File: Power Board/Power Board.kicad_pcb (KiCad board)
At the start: 2 copper layers, 55 x 70 mm, 147 parts, among them J1 Conn_02x07_Odd_Even, J2 Screw_Terminal_01x06, J3 Conn_01x03, J4 Conn_01x02, J5 Conn_02x03_Odd_Even, Q1 SI7157DP, Q2 SI7157DP, Q3 SI7157DP, Q4 SI7157DP, Q5 SI7157DP, Q6 SI7157DP, Q7 DMG2305UX, U1 LTC4417CGN, U10 LTC4150, U11 ATxmega32E5-AU, U2 TPS564208DDCT, U3 LTC3130-1, U4 LMR62014XMF, U5 TPS22810, U6 BQ2057WSNTR, U7 BQ29209DRBT, U8 LT6700CS6-1, U9 STS8C5H30L

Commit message: Started routing of blocks
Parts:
- moved C20 25.9 mm to (360.7, 181.1), turned to 90 degrees
- moved R25 20.9 mm to (360.7, 183.9), turned to 270 degrees
- moved R27 18.7 mm to (359.1, 183.9), turned to 90 degrees
- moved R26 18.1 mm to (371.1, 182.9), turned to 180 degrees
- moved D16 13.6 mm to (371.1, 184.3), turned to 180 degrees
- moved U6 13.2 mm to (365.5, 182.5)
- moved R24 12.8 mm to (363.3, 177.5), turned to 180 degrees
- moved Q7 10.0 mm to (369.3, 177.5), turned to 180 degrees
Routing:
- net /BAT_CELL_2: track 0.00 -> 9.93 mm
- net /BAT_CHARGE_VCC: track 0.00 -> 9.08 mm
- net Net-(Q7-Pad3): track 0.00 -> 7.43 mm
- net Net-(Q7-Pad1): track 0.00 -> 4.56 mm
- net Net-(J4-Pad1): track 0.00 -> 3.80 mm
- net /CHARGE_STAT: track 0.00 -> 2.14 mm
- net Net-(D16-Pad1): track 0.00 -> 1.42 mm

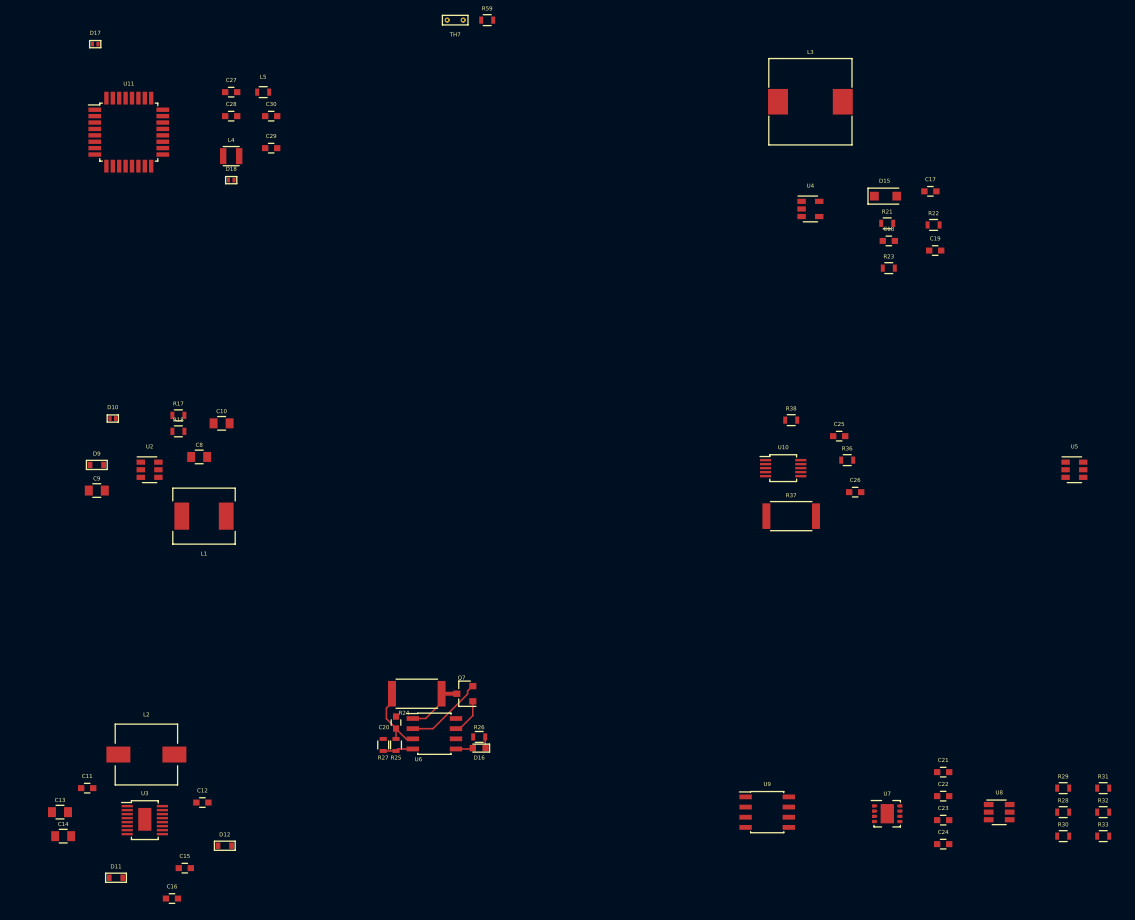
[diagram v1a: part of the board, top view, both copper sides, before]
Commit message: More blocks routed
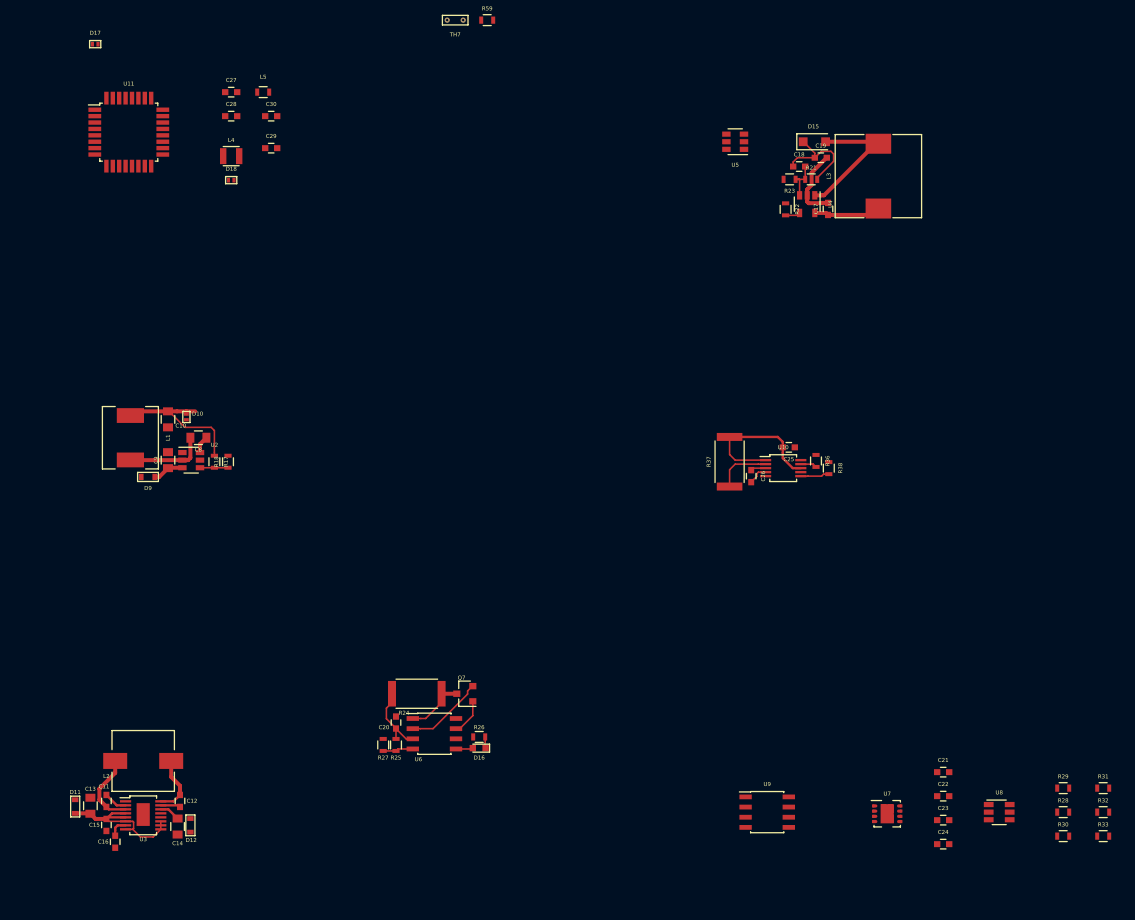
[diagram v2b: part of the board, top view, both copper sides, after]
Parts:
- moved U5 59.0 mm to (403.1, 108.5), turned to 180 degrees
- moved R22 18.6 mm to (409.4, 117.0), turned to 270 degrees
- moved C19 18.4 mm to (413.8, 110.5)
- moved R23 16.6 mm to (409.9, 113.2), turned to 180 degrees
- moved C18 14.6 mm to (411.1, 111.6)
- moved C14 14.4 mm to (333.4, 194.1), turned to 270 degrees
- moved L1 13.4 mm to (327.5, 145.5), turned to 90 degrees
- moved C26 13.2 mm to (405.1, 150.3), turned to 270 degrees
- moved C17 13.0 mm to (414.7, 116.9), turned to 90 degrees
- moved L3 12.6 mm to (421.0, 112.8), turned to 90 degrees
- moved D15 11.2 mm to (413.0, 108.5)
- moved C15 11.2 mm to (324.5, 193.9), turned to 270 degrees
- moved R21 11.0 mm to (412.6, 113.2)
- moved R37 10.3 mm to (402.4, 148.5), turned to 90 degrees
- moved D11 10.3 mm to (320.6, 191.6), turned to 90 degrees
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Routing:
- net /VCC_IN: track 0.00 -> 24.0 mm
- net /BAT_CELL_2: track 9.93 -> 28.6 mm
- net +3V3: track 0.00 -> 18.6 mm
- net Net-(D15-Pad2): track 0.00 -> 17.3 mm
- net Net-(C18-Pad1): track 0.00 -> 12.9 mm
- net Net-(C8-Pad2): track 0.00 -> 10.1 mm
- net Net-(C11-Pad2): track 0.00 -> 9.45 mm
- net GND: track 0.00 -> 9.22 mm
- net /UMB_VCC: track 0.00 -> 8.38 mm
- net Net-(C12-Pad1): track 0.00 -> 7.44 mm
- net /BAT_CELL_2_CONN: track 0.00 -> 6.89 mm
- net Net-(C18-Pad2): track 0.00 -> 5.27 mm
- net /LVL_POL: track 0.00 -> 3.60 mm
- net Net-(R17-Pad2): track 0.00 -> 3.50 mm
- net Net-(C11-Pad1): track 0.00 -> 2.94 mm
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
